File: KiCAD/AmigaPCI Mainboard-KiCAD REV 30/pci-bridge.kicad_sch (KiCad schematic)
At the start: 46 parts, among them CN109 SPI, CN110 SPI, U109 ICE40HX4K-TQ144, U109F1 W25X20CLSN, U110 ICE40HX4K-TQ144, U110F1 W25X20CLSN

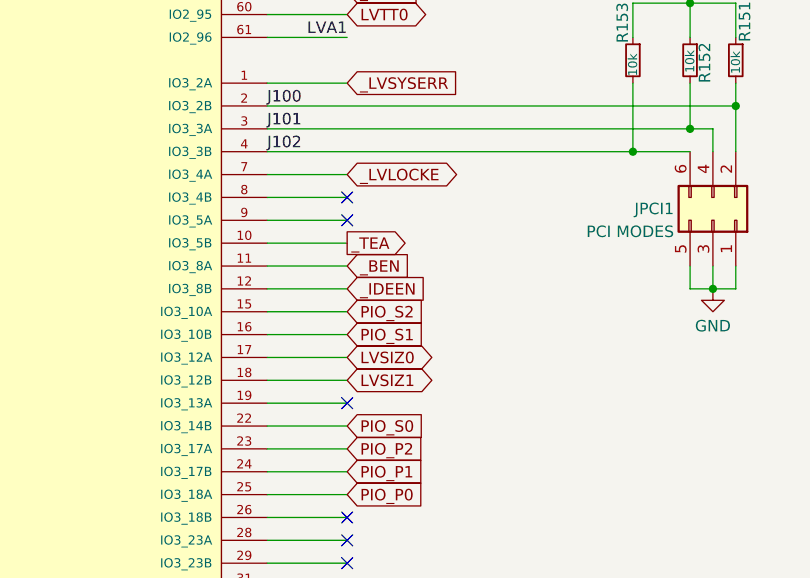
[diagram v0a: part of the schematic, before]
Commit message: Main Board Routing 22-May-2024a
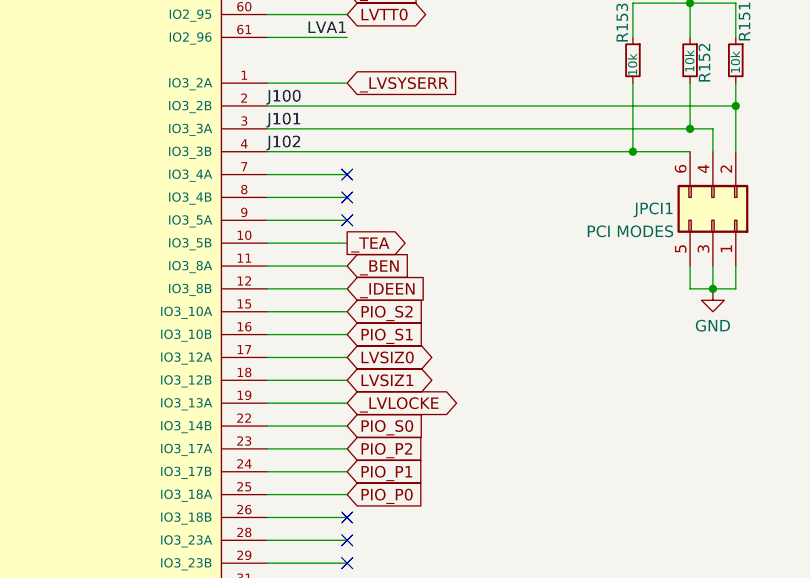
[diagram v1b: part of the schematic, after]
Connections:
- net _LVLOCKE: now also U110.19 (IO3_13A); no longer U110.7 (IO3_4A)
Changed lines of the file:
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@@
 	)
 	(no_connect
-		(at 281.94 187.96)
+		(at 281.94 162.56)
 	)
 	(no_connect
@@
 	(global_label "_LVLOCKE"
 		(shape bidirectional)
-		(at 281.94 162.56 0)
+		(at 281.94 187.96 0)
 		(fields_autoplaced yes)
 		(effects
@@
 		)
 		(property "Intersheetrefs" "${INTERSHEET_REFS}"
-			(at 295.1684 162.56 0)
+			(at 295.1684 187.96 0)
 			(effects
 				(font
